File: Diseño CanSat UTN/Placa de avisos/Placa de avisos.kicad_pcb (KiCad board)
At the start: 2 copper layers, 60 x 60 mm, 15 parts, among them J1 Conn_01x15_MountingPin, J2 Conn_01x15_MountingPin

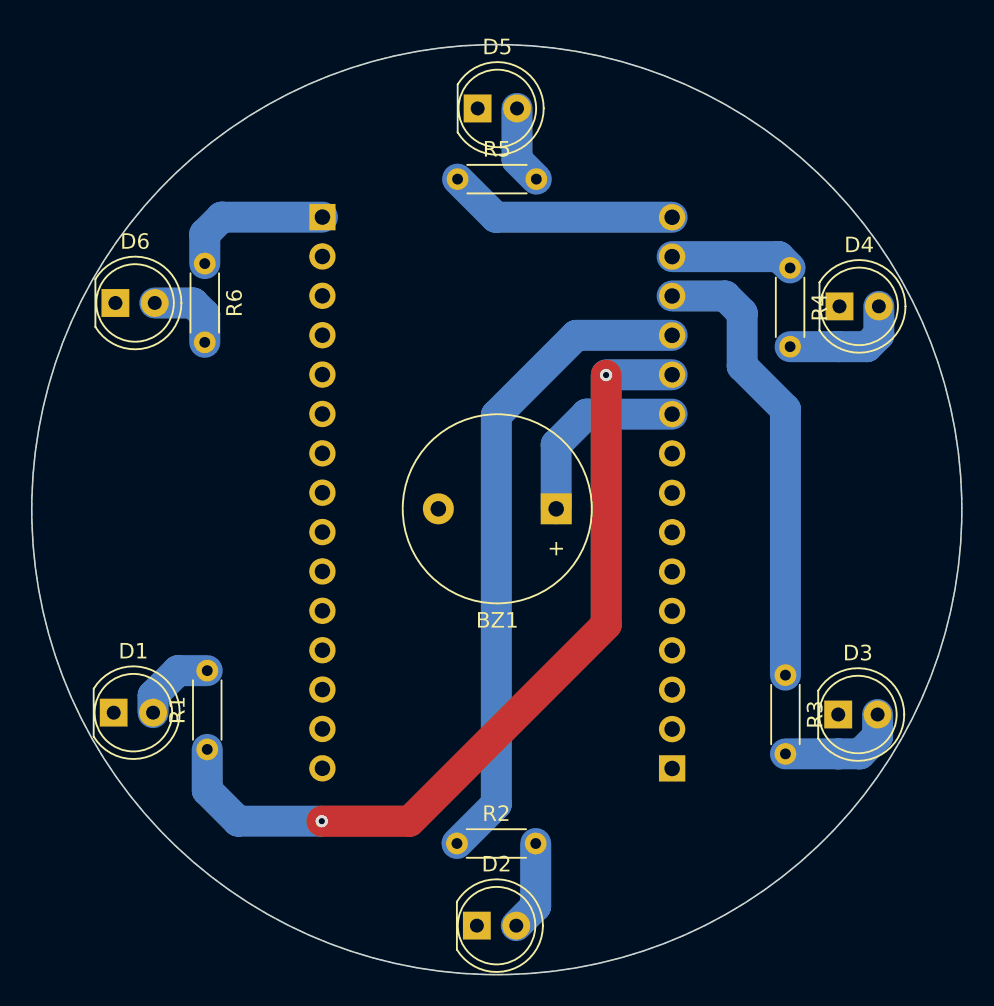
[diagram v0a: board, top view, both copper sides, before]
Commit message: ACTUALIZACION
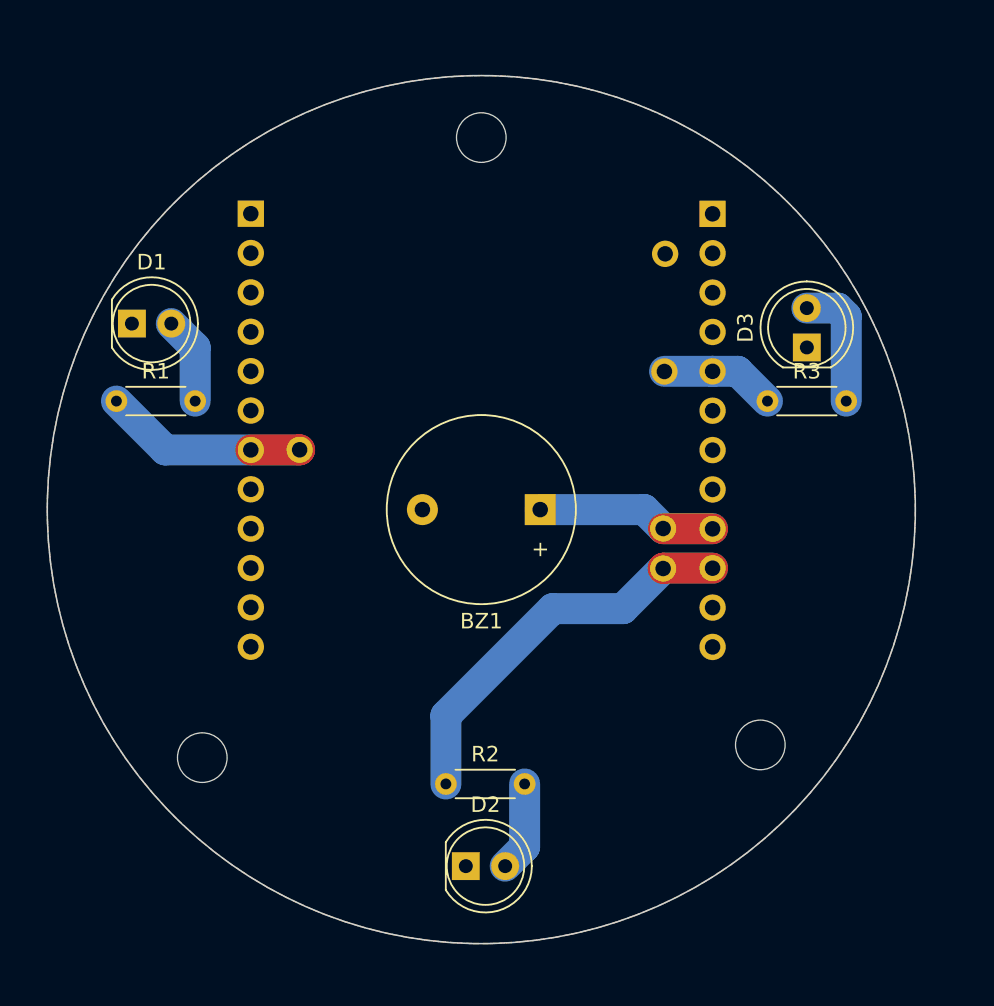
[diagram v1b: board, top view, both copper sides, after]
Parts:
- removed D4, D5, D6: LED, LED_THT:LED_D5.0mm
- removed R4, R5, R6: R, Resistor_THT:R_Axial_DIN0204_L3.6mm_D1.6mm_P5.08mm_Horizontal
- added ?: , , F.Cu at (160.8, 91.1)
- added ?: , , F.Cu at (160.7, 103.8)
- added ?: , , F.Cu at (160.9, 83.5)
- added ?: , , F.Cu at (160.7, 101.2)
- added ?: , , F.Cu at (137.3, 96.1)
- added REF**: MountingHole_3.2mm_M3, MountingHole:MountingHole_3.2mm_M3, F.Cu at (167.0, 115.2)
- added REF**: MountingHole_3.2mm_M3, MountingHole:MountingHole_3.2mm_M3, F.Cu at (149.0, 76.0)
- added REF**: MountingHole_3.2mm_M3, MountingHole:MountingHole_3.2mm_M3, F.Cu at (131.0, 116.0)
- moved J2 35.9 mm to (163.9, 80.9), turned to 180 degrees
- moved D1 25.1 mm to (126.5, 88.0)
- moved D3 23.8 mm to (170.0, 89.5), turned to 90 degrees
- moved R1 23.2 mm to (125.5, 93.0), turned to 0 degrees
- moved R3 17.7 mm to (167.5, 93.0), turned to 0 degrees
- moved J1 4.63 mm to (134.1, 80.9)
- moved D2 3.91 mm to (148.0, 123.0)
- moved R2 3.91 mm to (146.7, 117.7)
- moved BZ1 1.03 mm to (152.8, 100.0)
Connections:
- BZ1 pad 1: /10 -> /9
- J1 pad 4: /19 -> GND
- J2 pad 4: GND -> /4
- R1 pad 1: /11 -> /22
- R2 pad 1: /12 -> /10
- R3 pad 1: /13 -> /5
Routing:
- net /11: track 54.8 -> 0.13 mm, vias 2 -> 0
- net /12: track 42.2 -> 0.00 mm
- net /13: track 29.5 -> 0.00 mm
- net /10: track 12.4 -> 28.8 mm
- net /15: track 14.9 -> 0.00 mm
- net /9: track 0.00 -> 14.8 mm
- net /22: track 0.00 -> 13.1 mm
- net /16: track 9.95 -> 0.00 mm
- net /14: track 7.91 -> 0.00 mm
- net Net-(D4-A): track 7.88 -> 0.00 mm
- net /5: track 0.00 -> 7.45 mm
- net Net-(D6-A): track 5.33 -> 0.00 mm
- net Net-(D5-A): track 5.08 -> 0.00 mm
- added copper zone on F.Cu, net GND
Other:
- board size 60 x 60 mm -> 56 x 56 mm
